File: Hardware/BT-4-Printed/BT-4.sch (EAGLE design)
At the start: 78 parts, among them J1 CORTEX_DEBUG_PTH, J2 AVR_SPI_PROG_3X22X3_LOCK, J3 JST_ZH_2PIN, U1 ATMEGA1284P-AU, U2 TPS61200, U3 SIP32431DR3-T1GE3, U4 MAX40200AUK+, U5 MAX40200AUK+, U6 RFM95_96_97_98W, U7 XB5353A Ignore Pin Labels, U9 MICROCHIP_MCP1700T-3302E-TTMI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, Y1 CSTNE4M00GH5C000R0, Y3 TAXM8M4RFDCET2T

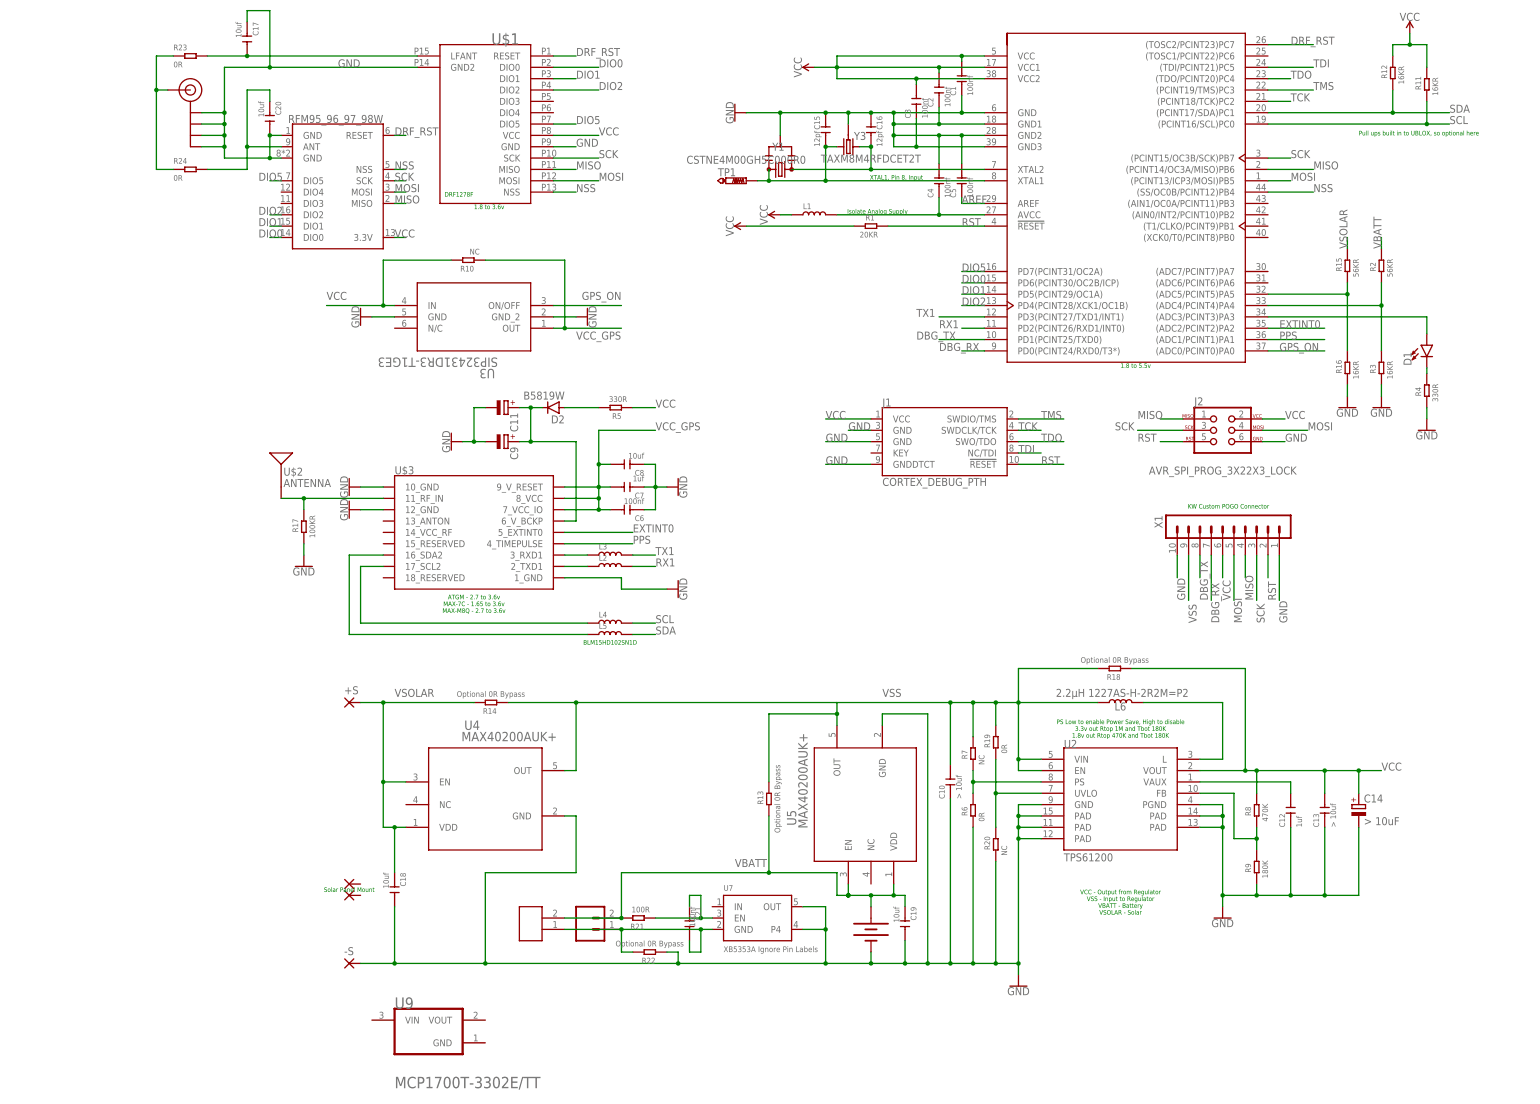
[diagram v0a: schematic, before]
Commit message: Sent to JLC
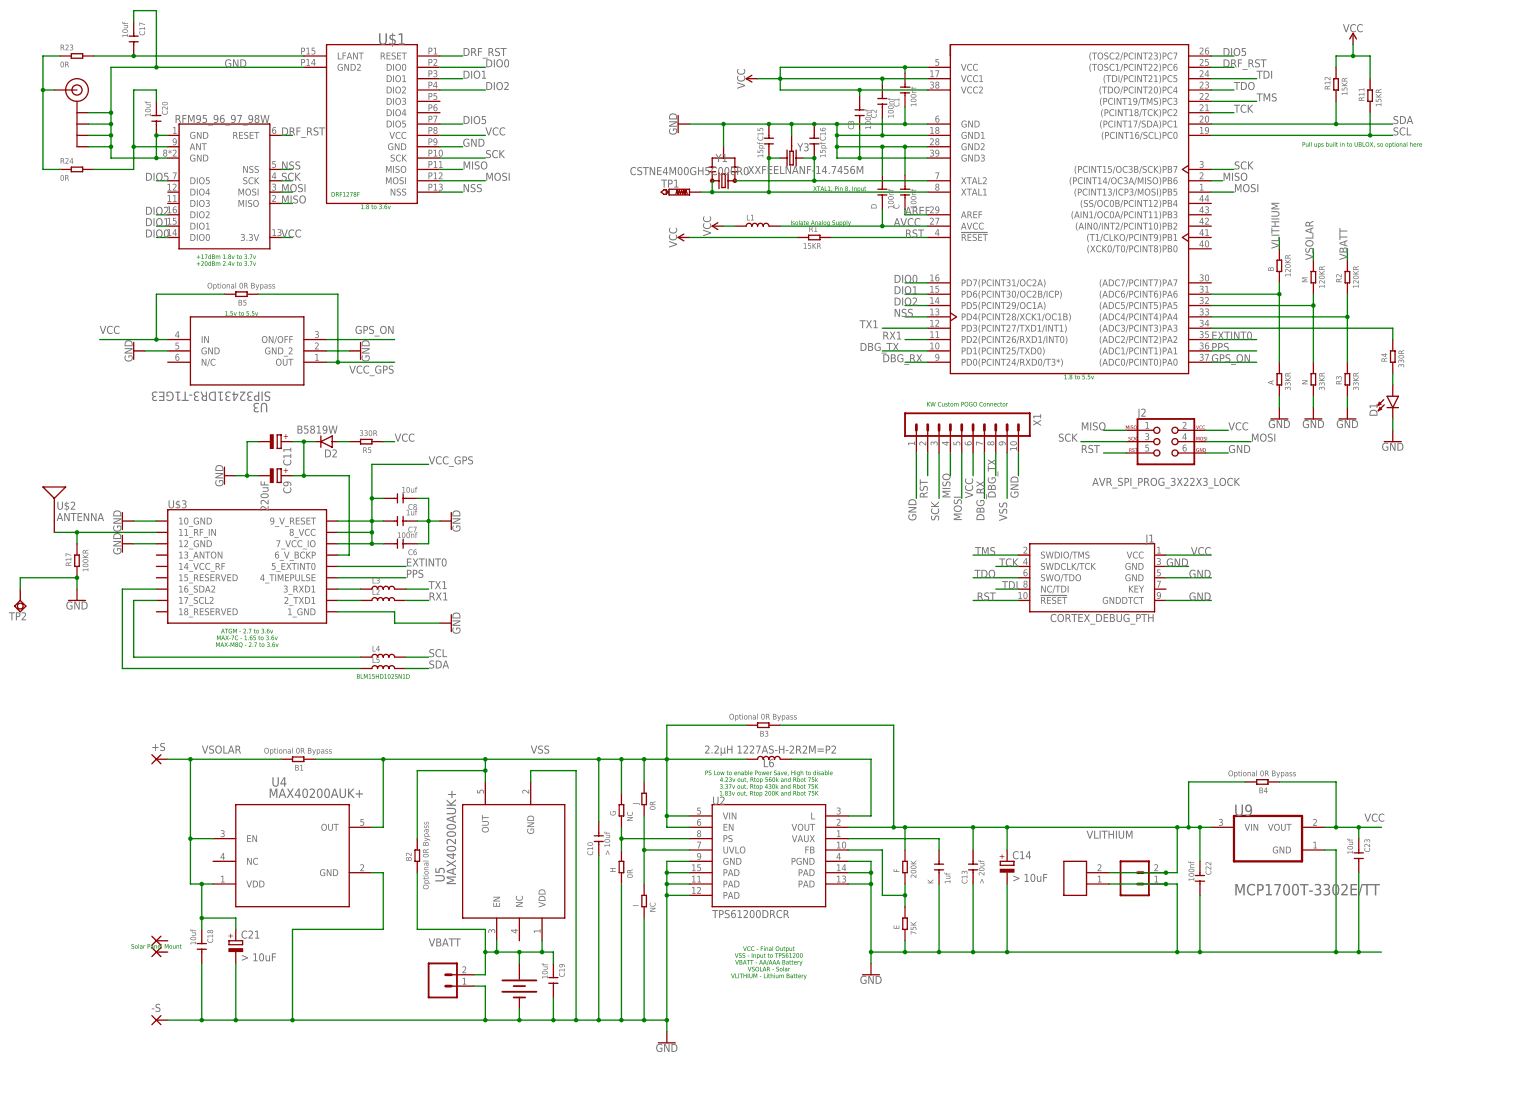
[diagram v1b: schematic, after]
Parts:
- removed C12: 1uf, OPL_Capacitor:CERAMIC-1UF-10V-10%-X5R(0402)
- removed C4, C5: 100nf, OPL_Capacitor:CERAMIC-100NF-25V-10%-X7R(0402)
- removed J3: JST_ZH_2PIN, ESP32-Cam-Pico-V4:JST_ZH_2PIN
- removed R10, R20, R7: NC, OPL_Resistor:SMD-RES-20K-5%-1/16W(0402)
- removed R13, R14, R18, R22: Optional 0R Bypass, OPL_Resistor:SMD-RES-20K-5%-1/16W(0402)
- removed R15: 56KR, OPL_Resistor:SMD-RES-20K-5%-1/16W(0402)
- removed R16: 16KR, OPL_Resistor:SMD-RES-20K-5%-1/16W(0402)
- removed R19, R6: 0R, OPL_Resistor:SMD-RES-20K-5%-1/16W(0402)
- removed R21: 100R, OPL_Resistor:SMD-RES-20K-5%-1/16W(0402)
- removed R8: 470K, OPL_Resistor:SMD-RES-20K-5%-1/16W(0402)
- removed R9: 180K, OPL_Resistor:SMD-RES-20K-5%-1/16W(0402)
- removed U7: XB5353A Ignore Pin Labels, Airquality_Sensor:VREG_SOT23-5
- added A, N: 33KR, OPL_Resistor:SMD-RES-20K-5%-1/16W(0402)
- added B, M: 120KR, OPL_Resistor:SMD-RES-20K-5%-1/16W(0402)
- added B1, B2, B3, B4, B5: Optional 0R Bypass, OPL_Resistor:SMD-RES-20K-5%-1/16W(0402)
- added C, C22, D: 100nf, OPL_Capacitor:CERAMIC-100NF-25V-10%-X7R(0402)
- added C23: 10uf, OPL_Capacitor:CERAMIC-10UF-6.3V-20%-X5R(0402)
- added E: 75K, OPL_Resistor:SMD-RES-20K-5%-1/16W(0402)
- added F: 200K, OPL_Resistor:SMD-RES-20K-5%-1/16W(0402)
- added G, I: NC, OPL_Resistor:SMD-RES-20K-5%-1/16W(0402)
- added H, J: 0R, OPL_Resistor:SMD-RES-20K-5%-1/16W(0402)
- added J5: JST_ZH_2PIN, ESP32-Cam-Pico-V4:JST_ZH_2PIN
- added J6: (no value), ESP32-Cam-Pico-V4:CONN_02JST-PTH-2-KIT
- added K: 1uf, OPL_Capacitor:CERAMIC-1UF-10V-10%-X5R(0402)
- added TP2: TPSQTP08SQ, testpad:TPSQTP08SQ
- C13: value > 10uf -> > 20uf
- C15, C16: value 12pf -> 15pf
- C21: value 100nf -> > 10uF; device OPL_Capacitor:CERAMIC-100NF-25V-10%-X7R(0402) -> KEW_HF_V16:RCL_CPOL-EUSMCC
- C9: value (none) -> 220uF
- D2: LCSC_PART (none) -> C8598
- L6: LCSC_PART (none) -> C435389
- R1: value 20KR -> 15KR
- R11, R12: value 16KR -> 15KR
- R2: value 56KR -> 120KR
- R3: value 16KR -> 33KR
- U1: LCSC_PART (none) -> C33575
- U2: value TPS61200 -> TPS61200DRCR; LCSC_PART (none) -> C140320
- U3: LCSC_PART (none) -> C141606
- Y3: value TAXM8M4RFDCET2T -> XXFEELNANF-14.7456M; LCSC_PART (none) -> C124311
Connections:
- net N$21 renamed L
- removed net N$17: R6.2, R7.1, U2.PS
- removed net N$18: C12.2, U2.VAUX
- removed net N$19: R8.1, R9.2, U2.FB
- removed net N$25: C21.2, J3.P$1, J4.1, R22.2, U7.GND
- removed net N$6: C4.1, L1.2, U1.AVCC
- removed net N$9: D1.C, R4.2
- new net AVCC: D.1, L1.2, U1.AVCC
- new net FB: E.2, F.1, U2.FB
- new net PS: G.1, H.2, U2.PS
- new net UVLO: I.2, J.1, U2.UVLO
- new net VAUX: K.2, U2.VAUX
- new net VLITHIUM: B.2, B3.1, B4.2, C13.2, C14.+, C22.1, F.2, J5.P$2, J6.2, U2.VOUT, U9.VIN
- net AREF: now also C.1; no longer C5.1
- net DIO0: now also U1.PD7(PCINT31/OC2A); no longer U1.PD6(PCINT30/OC2B/ICP)
- net DIO1: now also U1.PD6(PCINT30/OC2B/ICP); no longer U1.PD5(PCINT29/OC1A)
- net DIO2: now also U1.PD5(PCINT29/OC1A); no longer U1.PD4(PCINT28/XCK1/OC1B)
- net DIO5: now also U1.(TOSC2/PCINT23)PC7; no longer U1.PD7(PCINT31/OC2A)
- net DRF_RST: now also U1.(TOSC1/PCINT22)PC6; no longer U1.(TOSC2/PCINT23)PC7
- net GND: now also A.1, C.2, C21.-, C22.2, C23.2, D.2, D1.C, E.1, H.1, I.1, J4.1, J5.P$1, J6.1, K.1, N.1, TP2.TP, U9.GND; no longer C12.1, C4.2, C5.2, R16.1, R20.1, R22.1, R4.1, R6.1, R9.1, U7.OUT, U7.P4
- net N$2: now also D1.A, R4.1; no longer R19.1, R20.2, U2.UVLO
- net N$20: now also A.2, B.1, U1.(ADC6/PCINT6)PA6; no longer C21.1, R21.1, U7.EN
- net N$7: now also M.1, N.2; no longer R15.1, R16.2
- net N$8: now also R4.2; no longer D1.A
- net NSS: now also U1.PD4(PCINT28/XCK1/OC1B); no longer U1.(SS/OC0B/PCINT12)PB4
- net VBATT: now also B2.1; no longer J3.P$2, R13.1, R21.2
- net VCC: now also B4.1, B5.2, C23.1, U9.VOUT; no longer C13.2, C14.+, R10.2, R18.1, R8.2, U2.VOUT
- net VCC_GPS: now also B5.1; no longer R10.1
- net VSOLAR: now also B1.2, C21.+, M.2; no longer R14.2, R15.2
- net VSS: now also B1.1, B2.2, B3.2, G.2, J.2; no longer R13.2, R14.1, R18.2, R19.2, R7.2
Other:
- note added: "+17dBm 1.8v to 3.7v +20dBm 2.4v to 3.7v"
- note added: "1.5v to 5.5v"
- note added: "PS Low to enable Power Save, High to disable 4.23v out, Rtop 560k and Rbot 75k 3.37v out, Rtop 430k and Rbot 75K 1.83v out, Rtop 200K and Rbot 75K"
- note added: "VCC - Final Output VSS - Input to TPS61200 VBATT - AA/AAA Battery VSOLAR - Solar VLITHIUM - Lithium Battery"
- note removed: "PS Low to enable Power Save, High to disable 3.3v out Rtop 1M and Tbot 180K 1.8v out Rtop 470K and Tbot 180K"
- note removed: "VCC - Output from Regulator VSS - Input to Regulator VBATT - Battery VSOLAR - Solar"
- moved on the sheet: +S, -S, C1, C10, C11, C13, C14, C15, C16, C17, C18, C19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
